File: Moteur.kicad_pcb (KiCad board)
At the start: 4 copper layers, 31.7 x 16.1 mm, 53 parts, among them IC1 TPS71501, IC2 TLV710, IC3 MAX3051, IC4 LM5106, IC5 LM5106, IC6 INA282, P1 Bus2, P2 MOTOR, P3 GPIO, P4 CONN_1, P5 DBG, P6 CONN_1, Q1 IRF8721, Q2 IRF8721, Q3 IRF8721, Q4 IRF8721, U1 STM32F303CCT6, X1 16MHz

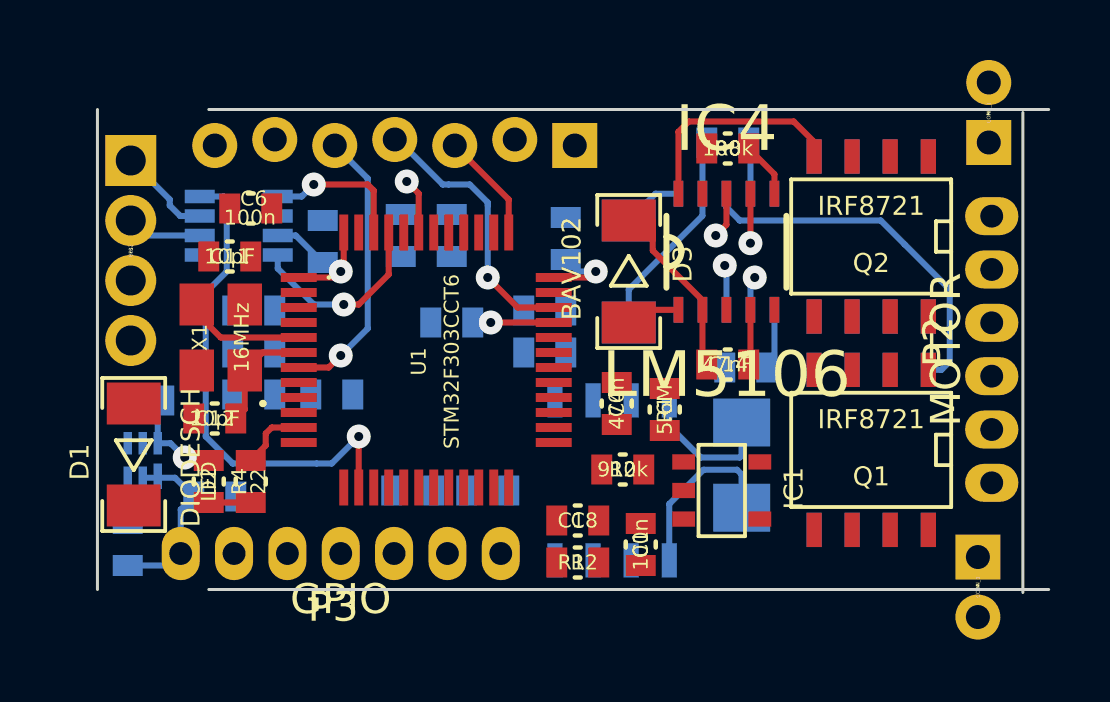
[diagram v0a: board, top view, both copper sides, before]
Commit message: routing (power)
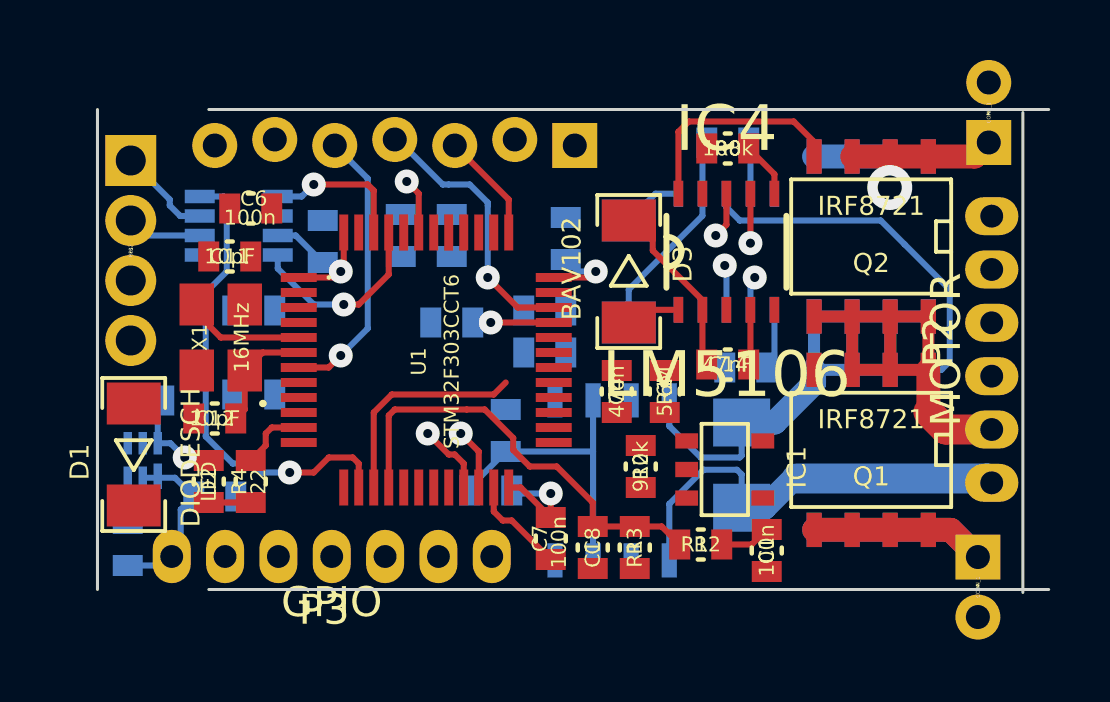
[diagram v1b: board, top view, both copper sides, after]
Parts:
- C7, R13: moved to F.Cu
- moved C8 8.79 mm to (135.9, 100.7), turned to 90 degrees
- moved R13 7.64 mm to (140.2, 104.6), turned to 270 degrees
- moved L1 6.19 mm to (135.4, 102.7)
- moved C1 4.20 mm to (144.6, 104.7), turned to 270 degrees
- moved R12 4.14 mm to (142.4, 104.5)
- moved C7 2.64 mm to (137.4, 104.3), turned to 270 degrees
- moved C18 1.03 mm to (138.8, 104.6), turned to 270 degrees
- moved IC1 0.71 mm to (143.2, 102.0)
- moved R2 0.61 mm to (140.4, 101.9), turned to 270 degrees
- moved R1 0.60 mm to (141.2, 99.4)
- moved C4 0.40 mm to (139.6, 99.4)
- moved P3 0.32 mm to (130.1, 104.9)
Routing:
- net Mot+: track 1.85 -> 18.1 mm
- net N-0000047: track 6.56 -> 21.6 mm
- net ADC/V_BAT: track 0.00 -> 14.7 mm
- net +BATT: track 0.00 -> 13.4 mm
- net GND: track 0.00 -> 12.7 mm, vias 0 -> 1
- net +3.3V_A: track 0.00 -> 10.0 mm
- net Mot-: track 5.94 -> 14.9 mm
- net ADC/I_MOT: track 0.00 -> 7.31 mm
- net +3.3V: track 11.5 -> 15.5 mm, vias 3 -> 4
- net Tx: track 0.00 -> 2.41 mm, vias 0 -> 1
- net Rx: track 0.00 -> 2.05 mm, vias 0 -> 1
- net CAN_SPEED: track 16.7 -> 15.8 mm
